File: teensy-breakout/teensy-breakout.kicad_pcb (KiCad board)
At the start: 6 copper layers, 139.7 x 133.4 mm, 90 parts, among them J1 USB_B, J10 Conn_01x04, J11 Conn_01x04, J12 Conn_01x05, J13 Conn_01x03, J14 Conn_01x04, J15 Conn_01x04, J16 Conn_01x02, J17 Conn_01x08, J18 Conn_01x08, J19 Conn_01x03, J2 Conn_01x02, J20 Conn_01x03, J21 Conn_01x03, J22 Conn_01x03, J3 Conn_01x02, J4 Conn_01x04, J5 Conn_01x04, J6 Conn_01x04, J7 Conn_01x04, J8 Conn_01x04, J9 Conn_01x04, Q1 IRL530NSTRLPBF, SW1 7101MD9AQE, U1 Teensy4.1, U10 LSF0102DCUR, U3 FT232RL, U6 ICL7667CBAZA-TDKR, U7 LSF0102DCUR

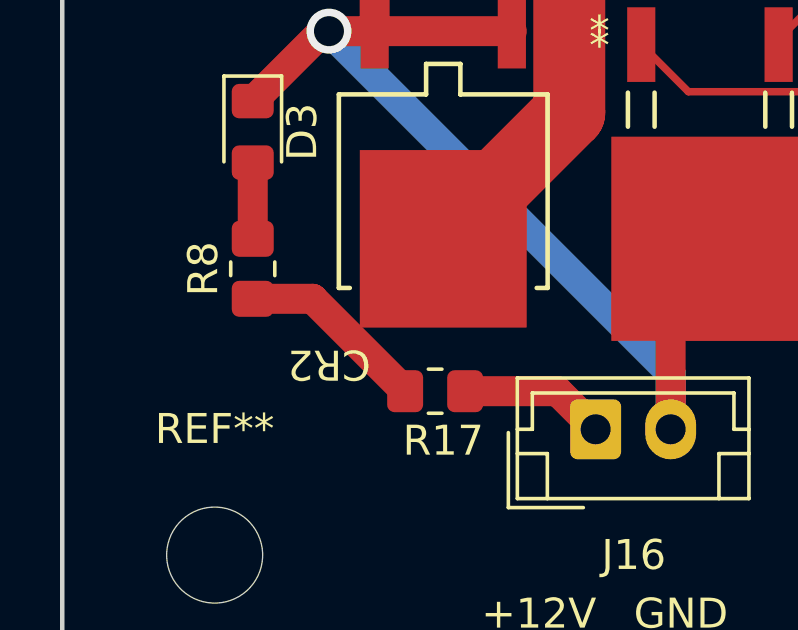
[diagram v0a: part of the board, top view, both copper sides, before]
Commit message: Fix small issue
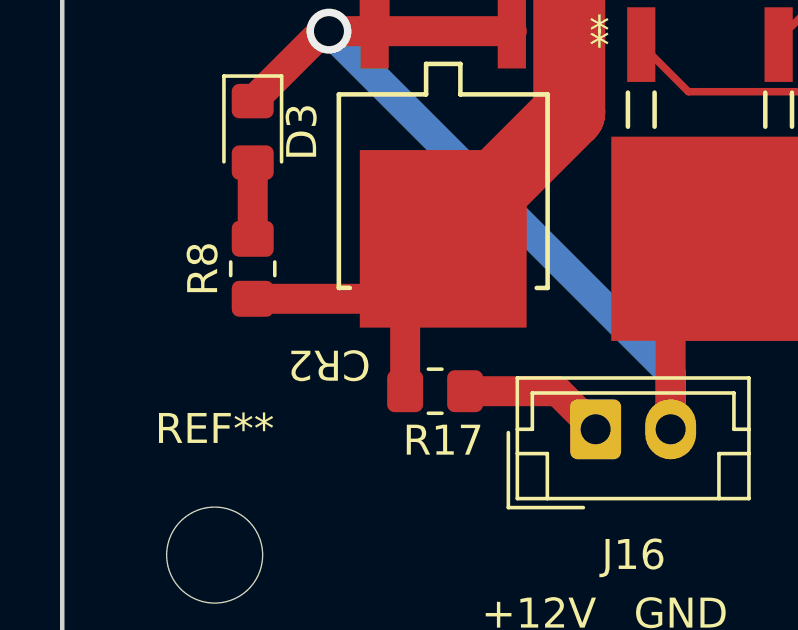
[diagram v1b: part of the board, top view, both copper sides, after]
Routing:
- net +12V: track 85.8 -> 92.3 mm
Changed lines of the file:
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@@
 	)
 	(segment
-		(start 105.41 253.077)
-		(end 107.41 253.077)
+		(start 109.76 253.077)
+		(end 111.76 251.077)
 		(width 1)
 		(layer "F.Cu")
@@
 	)
 	(segment
-		(start 107.41 253.077)
-		(end 110.49 256.157)
+		(start 105.41 253.077)
+		(end 109.76 253.077)
 		(width 1)
 		(layer "F.Cu")
@@
 	)
 	(segment
+		(start 110.49 256.157)
+		(end 110.49 252.347)
+		(width 1)
+		(layer "F.Cu")
+		(net 1)
+	)
+	(segment
 		(start 124.223718 212.09)
 		(end 123.19 212.09)
@@
 		(width 1)
 		(layer "F.Cu")
+		(net 1)
+	)
+	(segment
+		(start 110.49 252.347)
+		(end 111.76 251.077)
+		(width 1)
+		(layer "F.Cu")
